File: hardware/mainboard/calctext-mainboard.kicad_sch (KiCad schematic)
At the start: 36 parts, among them J1 LCD_FFC, J2 J_BAT+, J3 J_BAT-, SW1 Keypad_Contact, U1 Wio-E5-LE, U2 TPS61299, U3 PCAL9535APW,118

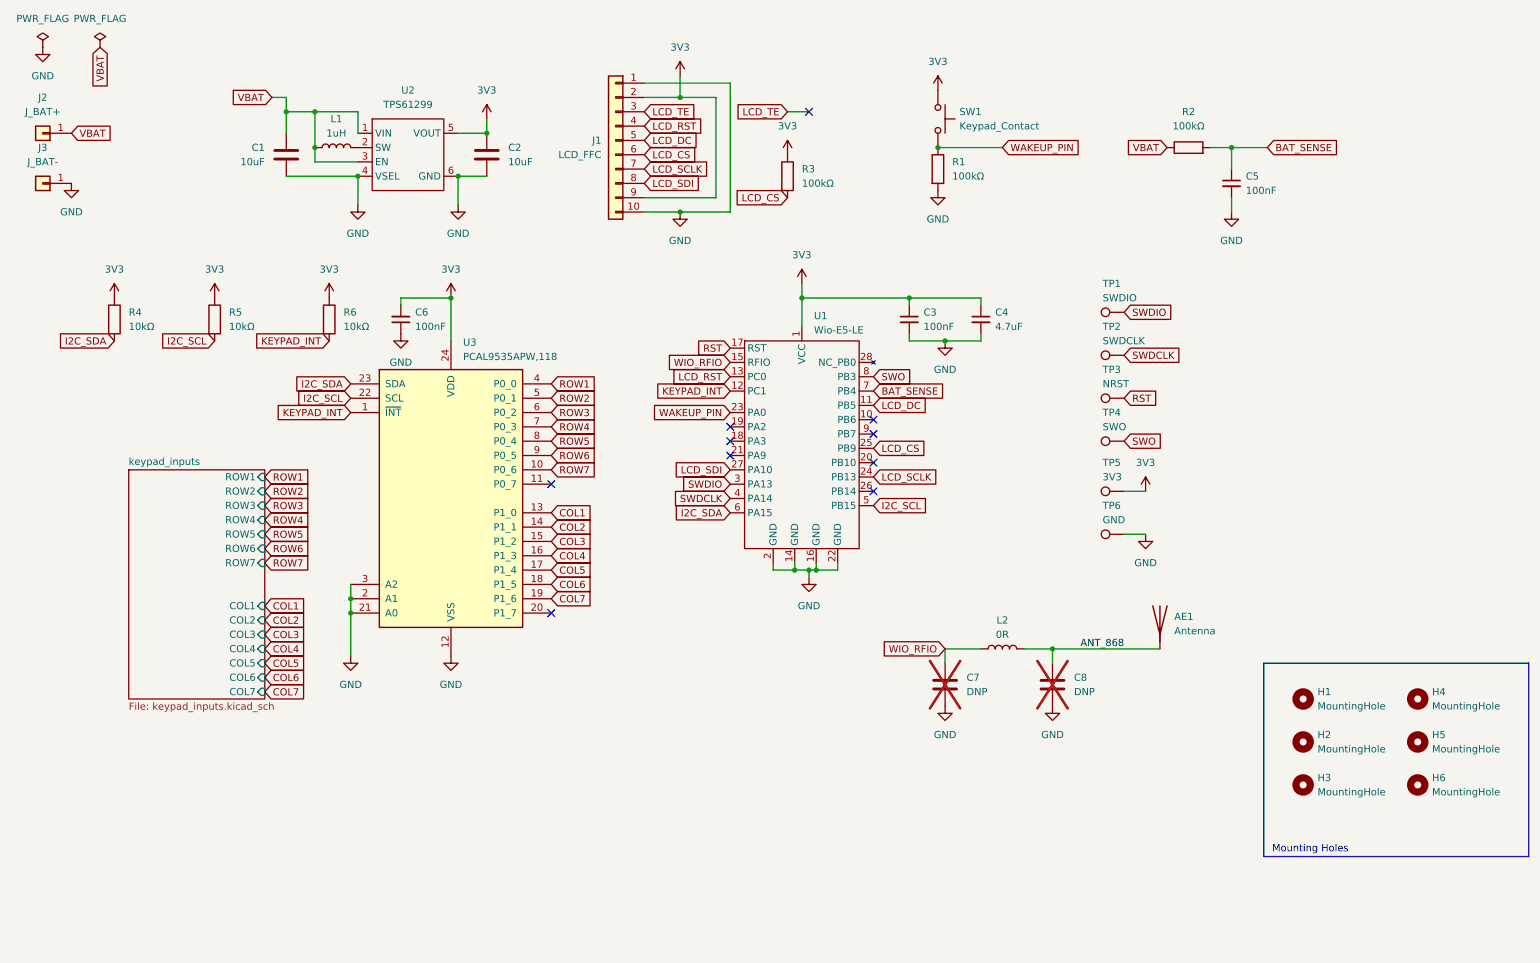
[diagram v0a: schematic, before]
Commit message: Polish mainboard schematic presentation
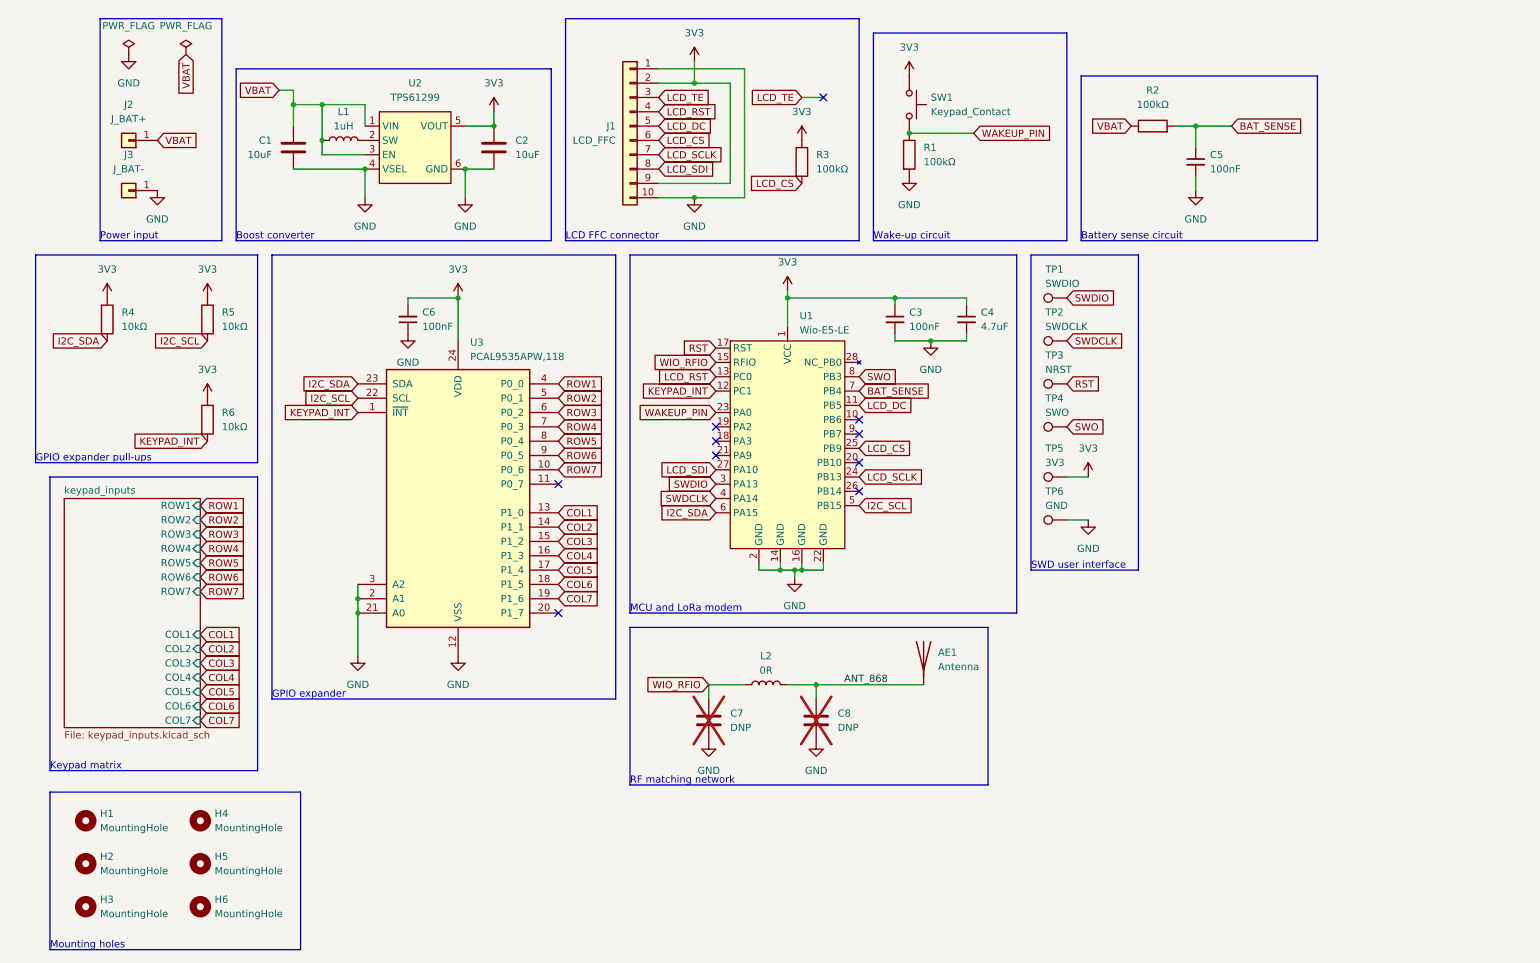
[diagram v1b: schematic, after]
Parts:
- U1: footprint CalcText:Wio-E5-LE -> Wio-E5-LE:Wio-E5-LE
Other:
- note added: "Battery sense circuit"
- note added: "Boost converter"
- note added: "GPIO expander"
- note added: "GPIO expander pull-ups"
- note added: "Keypad matrix"
- note added: "LCD FFC connector"
- note added: "MCU and LoRa modem"
- note added: "Mounting holes"
- note added: "Power input"
- note added: "RF matching network"
- note added: "SWD user interface"
- note added: "Wake-up circuit"
- note removed: "Mounting Holes"
- moved on the sheet: AE1, C1, C2, C3, C4, C5, C6, C7, C8, H1, H2, H3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
